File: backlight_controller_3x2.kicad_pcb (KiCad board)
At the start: 2 copper layers, 70.5 x 41.9 mm, 1 part

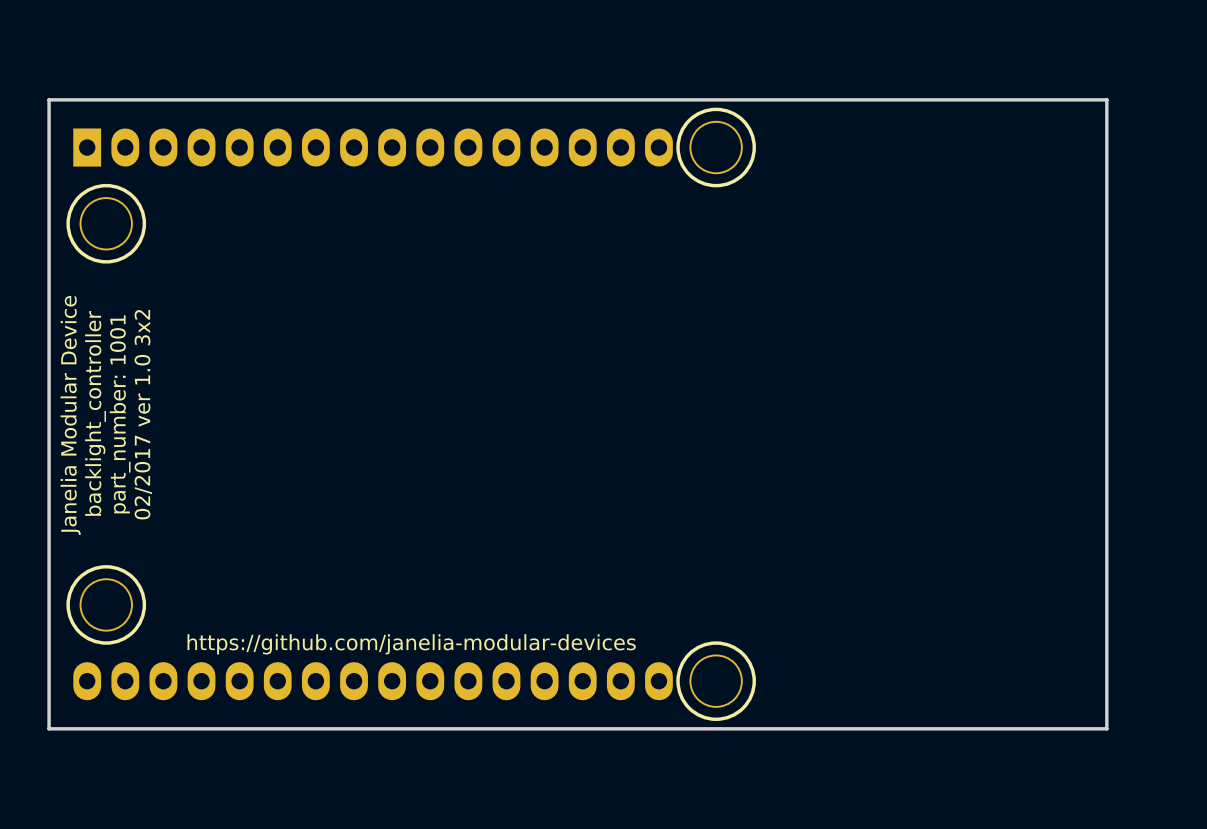
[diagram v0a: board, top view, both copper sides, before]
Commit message: Initial layout.
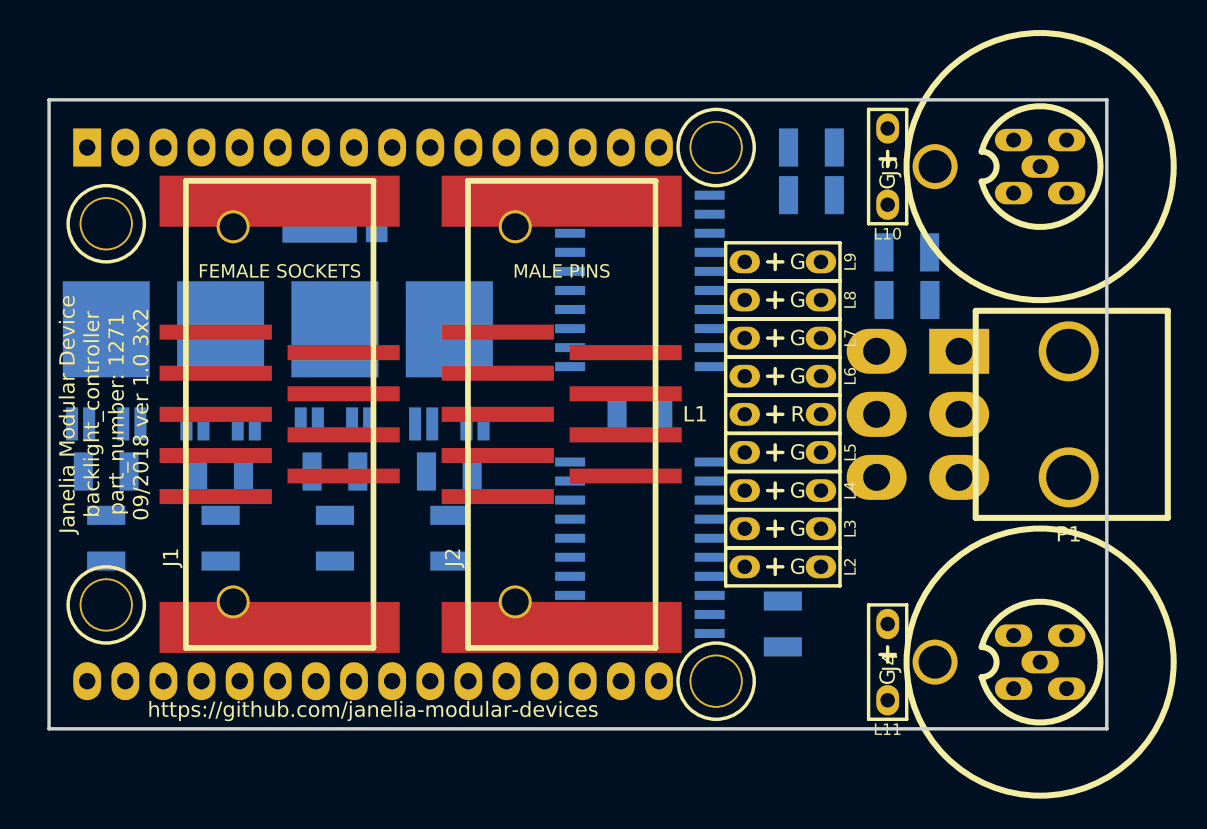
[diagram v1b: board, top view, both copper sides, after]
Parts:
- added C1: 0.1uF, backlight_controller_3x2:SM1210, B.Cu at (134.6, 102.9)
- added C2: 0.1uF, backlight_controller_3x2:SM1210, B.Cu at (125.1, 88.9)
- added C3: 0.1uF, backlight_controller_3x2:SM1210, B.Cu at (112.4, 92.7)
- added C4: 0.1uF, backlight_controller_3x2:SM1210, B.Cu at (104.8, 92.7)
- added C5: 0.1uF, backlight_controller_3x2:SM1210, B.Cu at (97.2, 92.7)
- added C6: 0.1uF, backlight_controller_3x2:SM1210, B.Cu at (89.5, 92.7)
- added D1: diode_schottky_45V_10A, backlight_controller_3x2:CFP15, B.Cu at (104.8, 75.6)
- added HPS1: BTS3256, backlight_controller_3x2:PG-TO252-5-11, B.Cu at (112.4, 89.5)
- added HPS2: BTS3256, backlight_controller_3x2:PG-TO252-5-11, B.Cu at (104.8, 89.5)
- added HPS3: BTS3256, backlight_controller_3x2:PG-TO252-5-11, B.Cu at (97.2, 89.5)
- added HPS4: BTS3256, backlight_controller_3x2:PG-TO252-5-11, B.Cu at (89.5, 89.5)
- added J1: DB9F_SMD, footprints:DB9F_SMD, F.Cu at (101.1, 88.9)
- added J2: DB9M_SMD, footprints:DB9M_SMD, F.Cu at (119.9, 88.9)
- added J3: M12-5_RCPT_F, backlight_controller_3x2:M12-5_RCPT_F, F.Cu at (151.8, 72.4)
- added J4: M12-5_RCPT_F, backlight_controller_3x2:M12-5_RCPT_F, F.Cu at (151.8, 105.4)
- added L1: LED_24V_RED, backlight_controller_3x2:LED_555-3XXX_R, F.Cu at (134.6, 88.9)
- added L10: LED_5V_GRN, backlight_controller_3x2:LED_555-3XXX_G, F.Cu at (141.6, 72.4)
- added L11: LED_5V_GRN, backlight_controller_3x2:LED_555-3XXX_G, F.Cu at (141.6, 105.4)
- added L2: LED_5V_GRN, backlight_controller_3x2:LED_555-3XXX_G, F.Cu at (134.6, 99.1)
- added L3: LED_5V_GRN, backlight_controller_3x2:LED_555-3XXX_G, F.Cu at (134.6, 96.5)
- added L4: LED_5V_GRN, backlight_controller_3x2:LED_555-3XXX_G, F.Cu at (134.6, 94.0)
- added L5: LED_5V_GRN, backlight_controller_3x2:LED_555-3XXX_G, F.Cu at (134.6, 91.4)
- added L6: LED_5V_GRN, backlight_controller_3x2:LED_555-3XXX_G, F.Cu at (134.6, 86.4)
- added L7: LED_5V_GRN, backlight_controller_3x2:LED_555-3XXX_G, F.Cu at (134.6, 83.8)
- added L8: LED_5V_GRN, backlight_controller_3x2:LED_555-3XXX_G, F.Cu at (134.6, 81.3)
- added L9: LED_5V_GRN, backlight_controller_3x2:LED_555-3XXX_G, F.Cu at (134.6, 78.7)
- added P1: MINI_FIT_JR_02X03_M_RA, backlight_controller_3x2:MINI-FIT-JR_02X03_M_RA, F.Cu at (153.7, 88.9)
- added R1: 5.9k, backlight_controller_3x2:SM1210, B.Cu at (112.4, 97.2)
- added R2: 5.9k, backlight_controller_3x2:SM1210, B.Cu at (104.8, 97.2)
- added R3: 5.9k, backlight_controller_3x2:SM1210, B.Cu at (97.2, 97.2)
- added R4: 5.9k, backlight_controller_3x2:SM1210, B.Cu at (89.5, 97.2)
- added R5: 140, backlight_controller_3x2:SM1210, B.Cu at (142.9, 81.3)
- added R6: 140, backlight_controller_3x2:SM1210, B.Cu at (142.9, 78.1)
- added R7: 140, backlight_controller_3x2:SM1210, B.Cu at (136.5, 74.3)
- added R8: 140, backlight_controller_3x2:SM1210, B.Cu at (136.5, 71.1)
- added U1: SN74ABT541BDWR, backlight_controller_3x2:SOIC_20, B.Cu at (125.1, 97.8)
- added U2: SN74ABT541BDWR, backlight_controller_3x2:SOIC_20, B.Cu at (125.1, 80.0)
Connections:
- MDB1 pad 14: (no net) -> /CHANNEL_4
- MDB1 pad 15: (no net) -> /CHANNEL_5
- MDB1 pad 16: (no net) -> /CHANNEL_6
- MDB1 pad 17: (no net) -> /CHANNEL_7
- MDB1 pad 18: (no net) -> /CHANNEL_8
- MDB1 pad 19: (no net) -> /CHANNEL_9
- MDB1 pad 2: (no net) -> /~ENABLE
- MDB1 pad 3: (no net) -> /CHANNEL_0
- MDB1 pad 4: (no net) -> /CHANNEL_1
- MDB1 pad 5: (no net) -> /CHANNEL_2
- MDB1 pad 6: (no net) -> /CHANNEL_3
- MDB1 pad GND: (no net) -> GND
- MDB1 pad VDD: (no net) -> VDD
- MDB1 pad VEE: (no net) -> VEE
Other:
- net class GND: trace_width 0.4064 -> 0.8128
- net class LEDPOWER: trace_width 0.6096 -> 0.4064
- board text added: "Janelia Modular Device backlight_controller part_number: 1271 09/2018 ver 1.0 3x2"
- board text removed: "Janelia Modular Device backlight_controller part_number: 1001 02/2017 ver 1.0 3x2"

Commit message: Finished version 1.0.
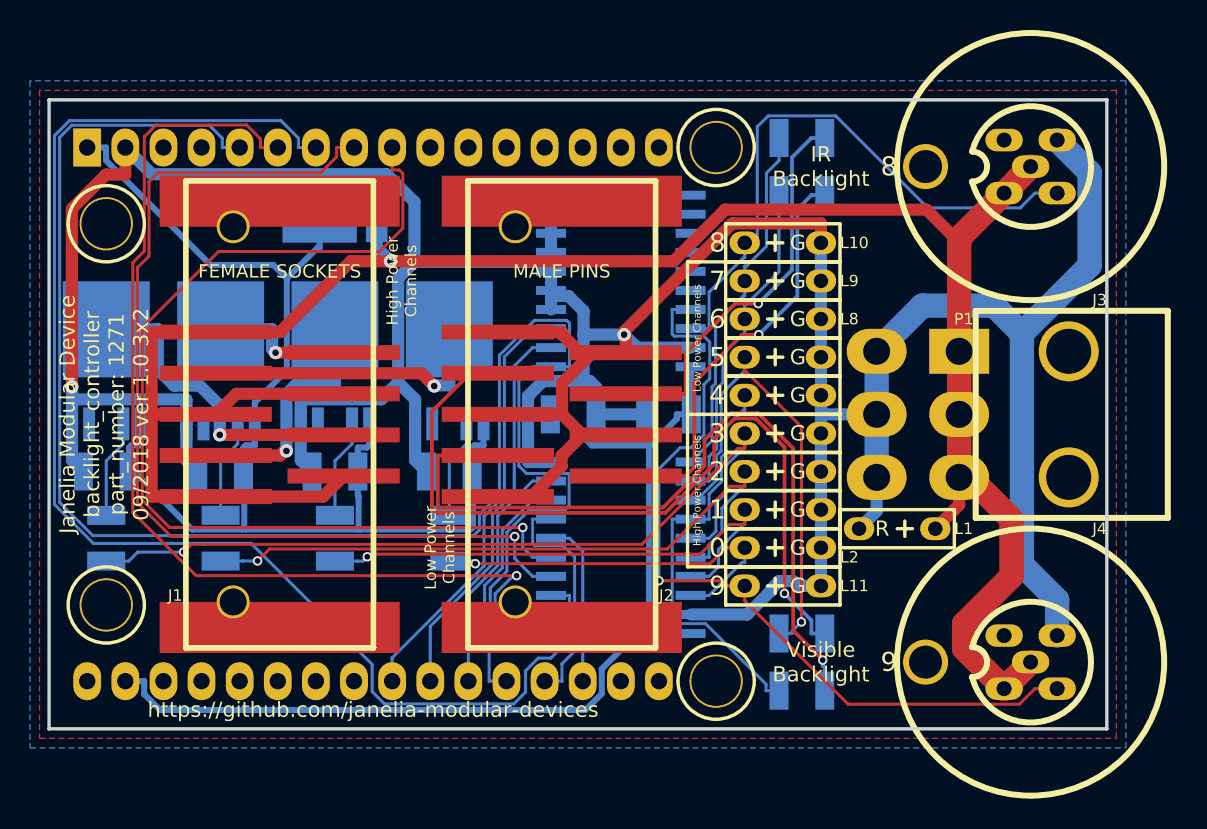
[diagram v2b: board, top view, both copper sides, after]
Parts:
- moved R5 27.0 mm to (135.9, 107.3), turned to 180 degrees
- moved R6 26.3 mm to (135.9, 103.5), turned to 180 degrees
- moved C1 19.8 mm to (120.7, 88.9), turned to 0 degrees
- moved L1 10.8 mm to (142.2, 96.5), turned to 270 degrees
- moved L10 8.64 mm to (134.6, 77.5), turned to 90 degrees
- moved L11 8.64 mm to (134.6, 100.3), turned to 90 degrees
- moved C2 1.91 mm to (127.0, 88.9)
- moved L4 1.27 mm to (134.6, 92.7)
- moved L7 1.27 mm to (134.6, 85.1)
- moved L9 1.27 mm to (134.6, 80.0)
- moved L2 1.27 mm to (134.6, 97.8)
- moved L3 1.27 mm to (134.6, 95.2)
- moved L5 1.27 mm to (134.6, 90.2)
- moved L6 1.27 mm to (134.6, 87.6)
- moved L8 1.27 mm to (134.6, 82.5)
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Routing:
- net GND: track 0.00 -> 283.2 mm, vias 0 -> 2
- net VAA: track 0.00 -> 149.3 mm, vias 0 -> 1
- net /~ENABLE: track 0.00 -> 117.9 mm
- net /CHANNEL_1: track 0.00 -> 91.2 mm
- net VDD: track 0.00 -> 84.8 mm
- net /CHANNEL_0: track 0.00 -> 70.1 mm, vias 0 -> 1
- net VEE: track 0.00 -> 69.2 mm
- net /CHANNEL_3: track 0.00 -> 67.1 mm, vias 0 -> 1
- net /CHANNEL_2: track 0.00 -> 67.1 mm, vias 0 -> 1
- net /backlight_3x2/C_3: track 0.00 -> 55.9 mm, vias 0 -> 1
- net /backlight_3x2/C_9: track 0.00 -> 54.3 mm, vias 0 -> 1
- net /backlight_3x2/low_power_outputs/OUTPUT_1: track 0.00 -> 54.0 mm, vias 0 -> 1
- net /backlight_3x2/low_power_outputs/OUTPUT_0: track 0.00 -> 52.7 mm, vias 0 -> 1
- net /backlight_3x2/C_2: track 0.00 -> 45.9 mm, vias 0 -> 1
- net /backlight_3x2/C_8: track 0.00 -> 39.8 mm
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- added copper zone on B.Cu, net GND
- added copper zone on F.Cu, net VAA
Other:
- net class LEDPOWER: clearance 0.254 -> 0.1016; trace_width 0.4064 -> 0.254; via_dia 0.889 -> 0.635; via_drill 0.635 -> 0.381
- net class POWER: clearance 0.254 -> 0.1016; trace_width 0.8128 -> 0.4064
- net class SIGNAL: trace_width 0.4064 -> 0.2032; via_dia 0.889 -> 0.635; via_drill 0.635 -> 0.381
- net class SUPERPOWER: clearance 0.254 -> 0.1016; trace_width 1.2192 -> 0.8128
- rule trace_min: 0.254 -> 0.2032
- rule via_min_drill: 0.508 -> 0.2032
- rule via_min_size: 0.889 -> 0.508
- board text added: "0"
- board text added: "1"
- board text added: "2"
- board text added: "3"
- board text added: "4"
- board text added: "5"
- board text added: "6"
- board text added: "7"
- board text added: "8"
- board text added: "9"
- board text added: "High Power Channels"
- board text added: "IR Backlight"
- board text added: "Low Power Channels"
- board text added: "Visible Backlight"
